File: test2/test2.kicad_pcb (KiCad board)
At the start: 2 copper layers, 5 parts, among them J1 USB_B_Micro, X1 Badgelife_sao_connector_v169b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

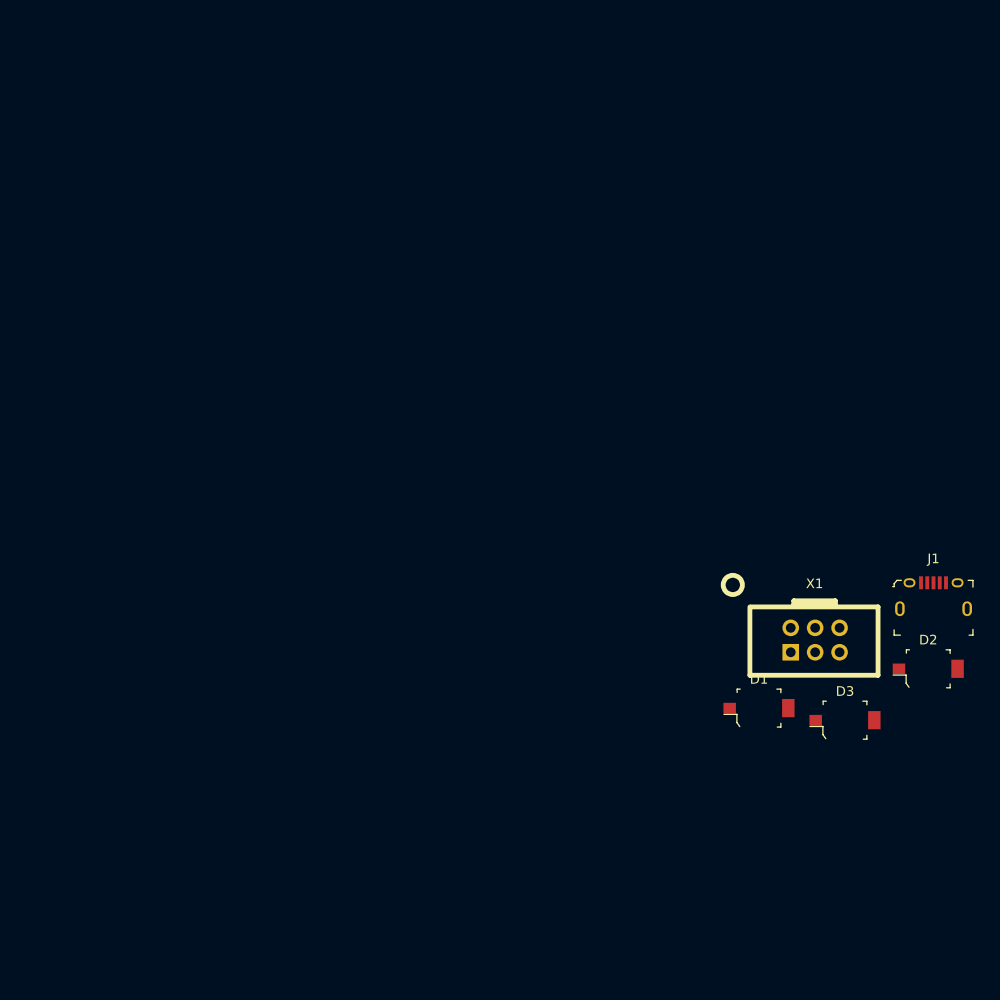
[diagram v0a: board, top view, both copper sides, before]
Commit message: .
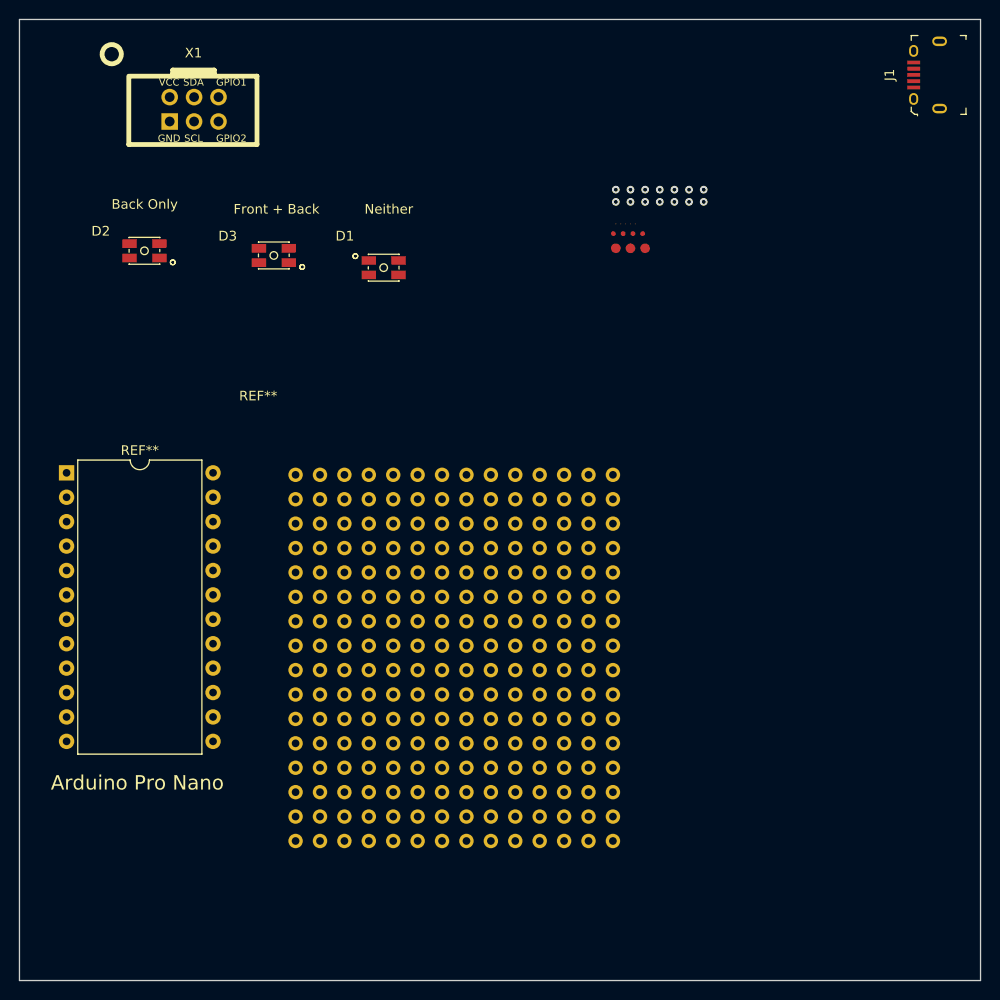
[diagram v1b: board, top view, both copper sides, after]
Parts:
- added REF**: ProtoBoard, test2:ProtoBoard, F.Cu at (91.9, 88.9)
- added REF**: dot, test2:dot, F.Cu at (130.8, 66.5)
- added REF**: dot, test2:dot, F.Cu at (130.3, 66.5)
- added REF**: dot, test2:dot, F.Cu at (129.8, 66.5)
- added REF**: dot, test2:dot, F.Cu at (129.3, 66.5)
- added REF**: dot, test2:dot, F.Cu at (128.8, 66.5)
- added REF**: DIP-24_W15.24mm, Package_DIP:DIP-24_W15.24mm, F.Cu at (71.6, 92.5)
- added REF**: dot-1mm, test2:dot-1mm, F.Cu at (131.8, 69.1)
- added REF**: dot-1mm, test2:dot-1mm, F.Cu at (130.3, 69.1)
- added REF**: dot-1mm, test2:dot-1mm, F.Cu at (128.8, 69.1)
- added REF**: dot-0.5mm, test2:dot-0.5mm, F.Cu at (131.6, 67.6)
- added REF**: dot-0.5mm, test2:dot-0.5mm, F.Cu at (130.6, 67.6)
- added REF**: dot-0.5mm, test2:dot-0.5mm, F.Cu at (129.5, 67.6)
- added REF**: dot-0.5mm, test2:dot-0.5mm, F.Cu at (128.5, 67.6)
- D1, D2, D3: footprint digikey-footprints:LED_2-SMD_Gull_Wing_4.4x3.85mm -> plcc4:MF_LEDs-PLCC4
- moved D2 92.4 mm to (79.7, 69.4), turned to 180 degrees
- moved X1 85.0 mm to (84.8, 54.6)
- moved D3 76.6 mm to (93.2, 69.8), turned to 180 degrees
- moved D1 60.2 mm to (104.6, 71.1)
- moved J1 52.9 mm to (159.8, 51.1), turned to 90 degrees
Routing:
- net (no net): vias 0 -> 14
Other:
- board outline added: 100 x 100 mm
- board text added: "Arduino Pro Nano"
- board text added: "Back Only"
- board text added: "Front + Back"
- board text added: "Neither"
